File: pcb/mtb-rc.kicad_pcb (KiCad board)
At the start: 4 copper layers, 100 x 70 mm, 166 parts, among them J1 MVE252-5-V, J10 MVE252-5-V, J11 MVE252-5-V, J2 MVE252-5-V, J3 MVE252-5-V, J4 MVE252-5-V, J5 MVE252-5-V, J6 PINHEADER, J7 PINHEADER, J8 PROG/DEBUG, J9 MVE252-5-V, SW1 6x6, U1 VO0631T, U10 LM339, U11 LM339, U12 STM32F103C8Tx, U13 HT7533-1, U14 78M05, U15 MAX487, U2 VO0631T, U3 VO0631T, U4 L78L05_SOT89, U5 L79L05_SOT89, U6 LM339, U7 LM339, U8 LM339, U9 4052, Y1 14.7456MHz

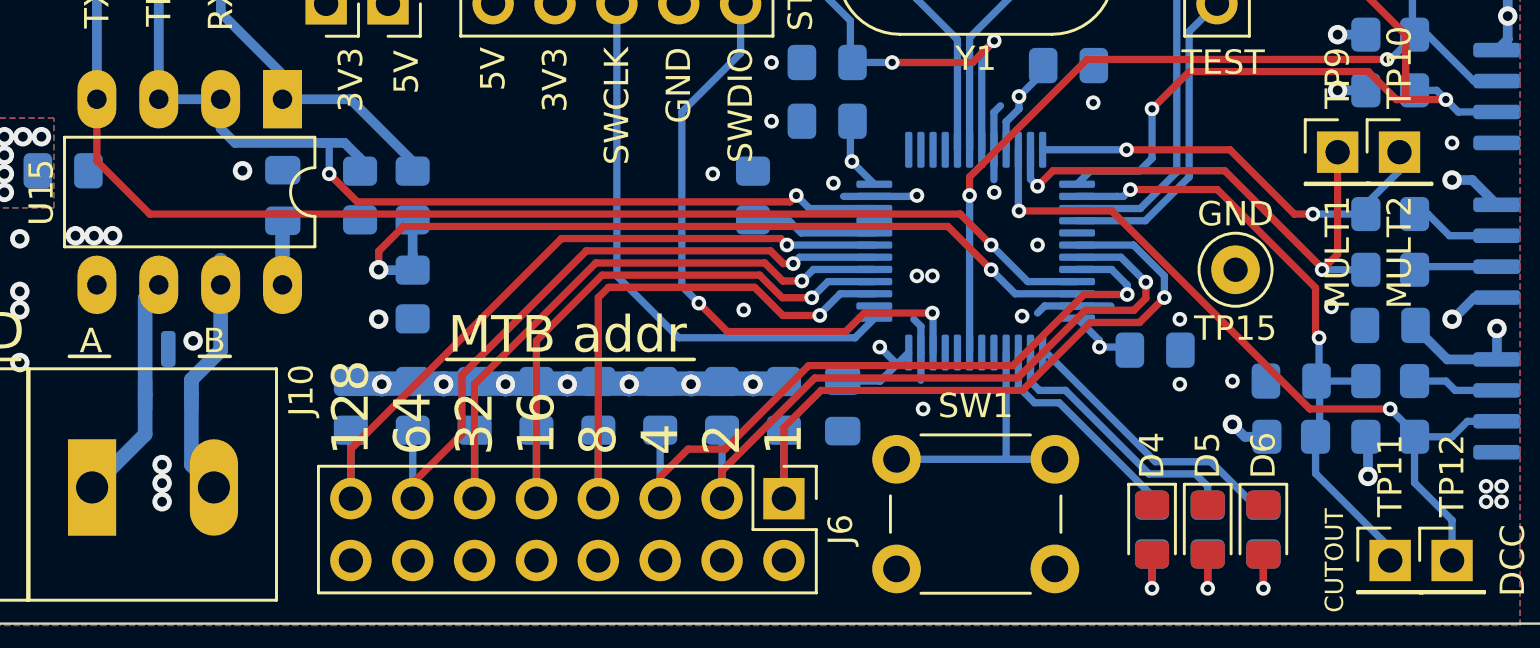
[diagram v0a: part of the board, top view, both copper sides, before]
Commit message: Minor tweaks.
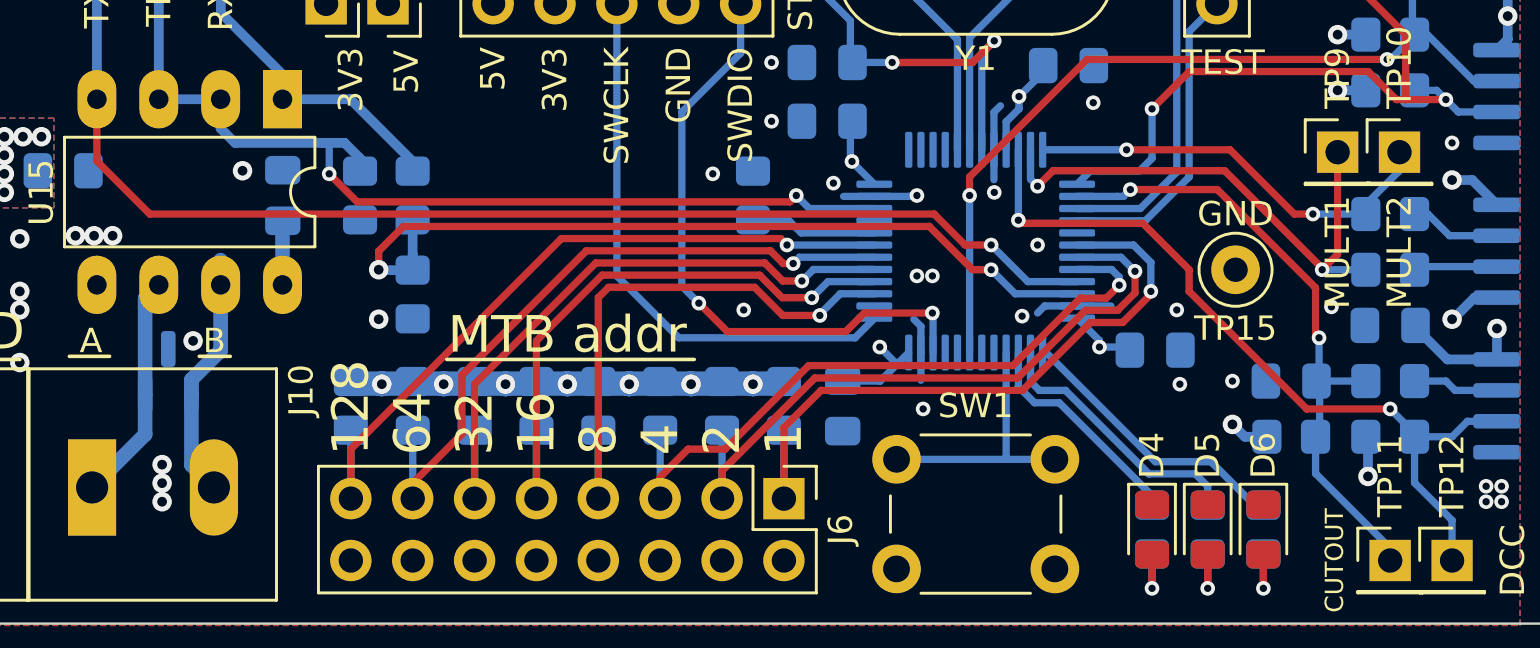
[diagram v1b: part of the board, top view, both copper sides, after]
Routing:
- net ADDR-1: track 28.6 -> 27.8 mm
- net /MTB/DCC: track 32.1 -> 32.9 mm
- net ADDR-2: track 28.3 -> 27.5 mm
- net ADDR-4: track 28.8 -> 28.1 mm
